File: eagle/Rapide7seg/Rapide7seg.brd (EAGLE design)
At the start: 50 x 50 mm, 47 parts, among them IC1 MEGA8-P, J1 AVR_SPI_PRG_6PTH

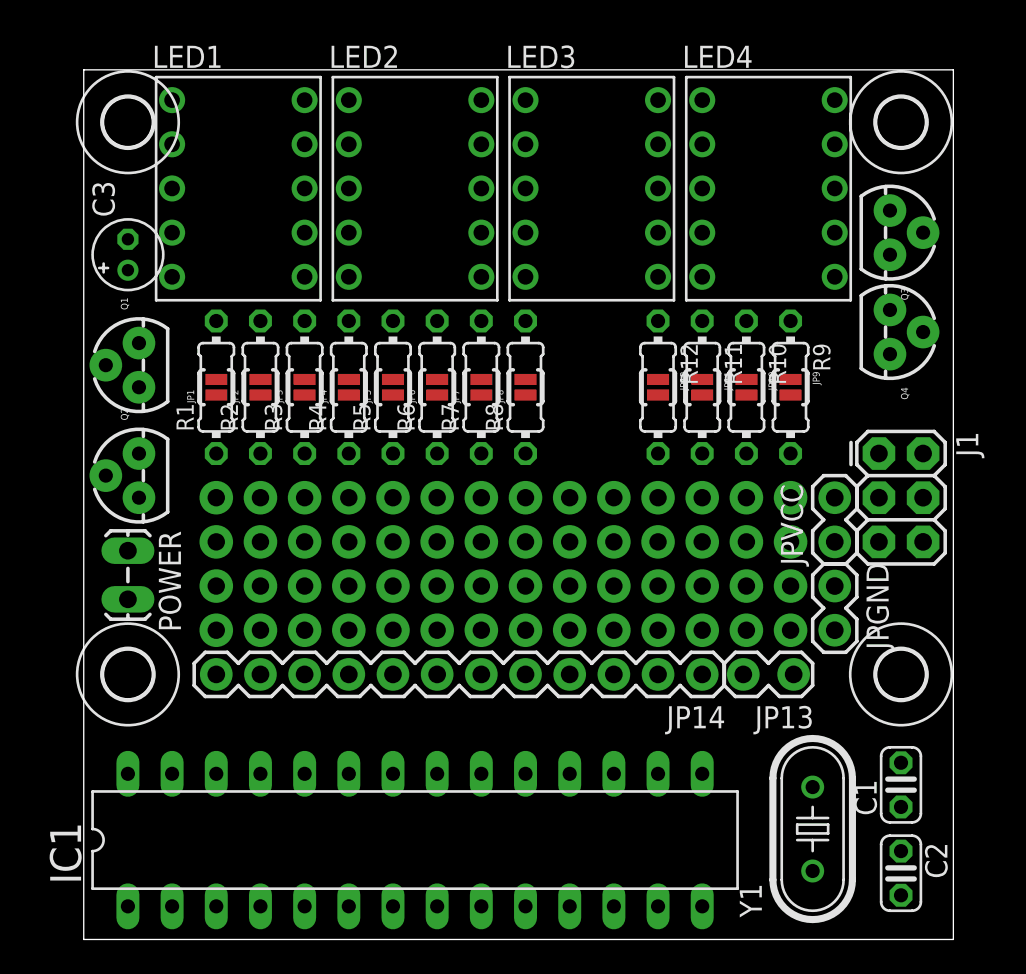
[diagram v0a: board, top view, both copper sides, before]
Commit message: First version, sent to production
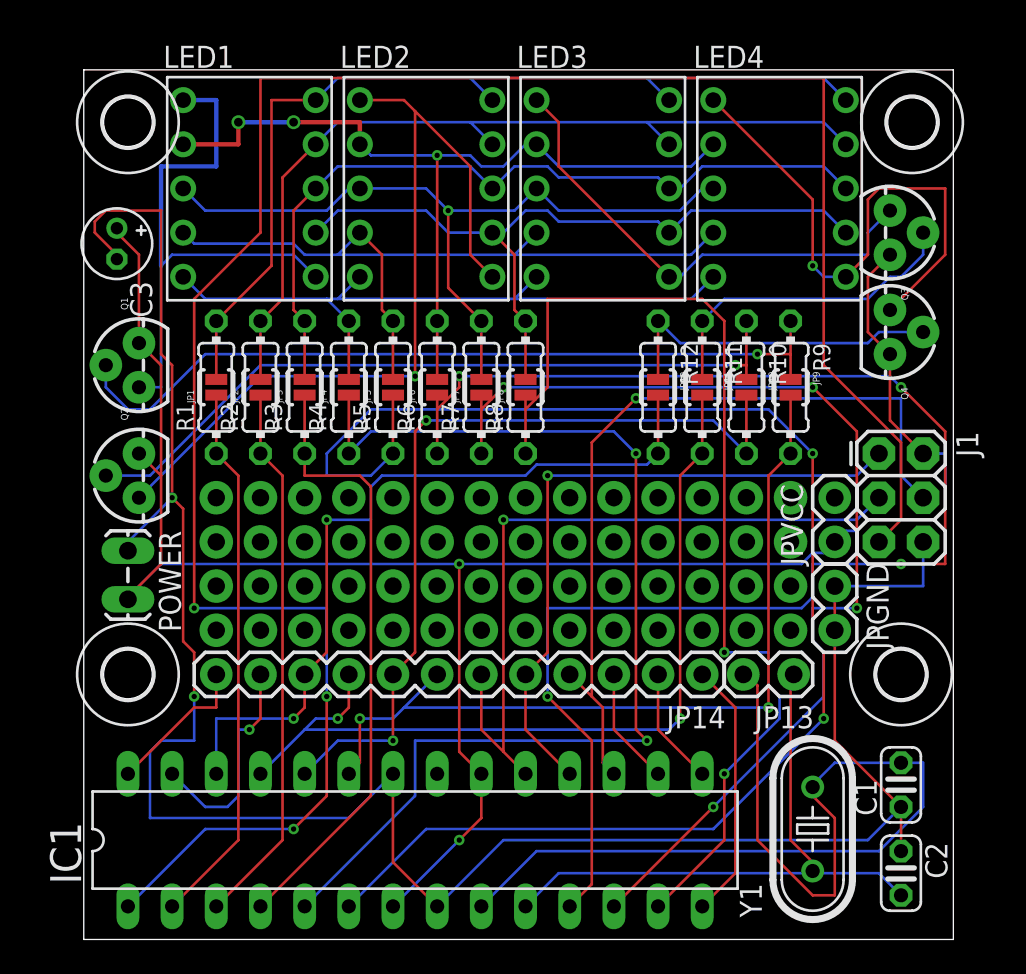
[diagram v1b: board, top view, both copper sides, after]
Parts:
- moved C3 0.90 mm to (1.91, 40.0), turned to 270 degrees
- moved LED4 0.64 mm to (40.0, 43.2)
- moved LED1 0.63 mm to (9.53, 43.2)
- moved H1 0.63 mm to (47.6, 47.0)
- moved LED2 0.63 mm to (19.7, 43.2)
- moved LED3 0.63 mm to (29.8, 43.2)
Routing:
- net UCRESET: track 0.00 -> 126.0 mm, vias 0 -> 3
- net GND: track 0.00 -> 125.9 mm, vias 0 -> 2
- net VCC: track 0.00 -> 114.2 mm, vias 0 -> 2
- net N$21: track 0.00 -> 86.4 mm, vias 0 -> 4
- net N$23: track 0.00 -> 86.3 mm, vias 0 -> 2
- net N$16: track 0.00 -> 63.2 mm, vias 0 -> 2
- net N$19: track 0.00 -> 61.6 mm, vias 0 -> 4
- net N$17: track 0.00 -> 60.3 mm, vias 0 -> 2
- net N$1: track 0.00 -> 59.8 mm
- net N$9: track 0.00 -> 55.0 mm
- net N$11: track 0.00 -> 50.0 mm
- net L3: track 0.00 -> 49.5 mm, vias 0 -> 2
- net N$26: track 0.00 -> 48.8 mm, vias 0 -> 1
- net L1: track 0.00 -> 48.4 mm, vias 0 -> 2
- net N$22: track 0.00 -> 48.0 mm, vias 0 -> 3
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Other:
- board text removed: "Order #######"
